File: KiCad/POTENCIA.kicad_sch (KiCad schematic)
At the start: 25 parts, among them J2 Screw_Terminal_01x02, J3 Screw_Terminal_01x02, J6 Screw_Terminal_01x02, SW7 SW_SPST, U2 LM2596S-5, U3 L298N, U7 LM1117DT-3.3

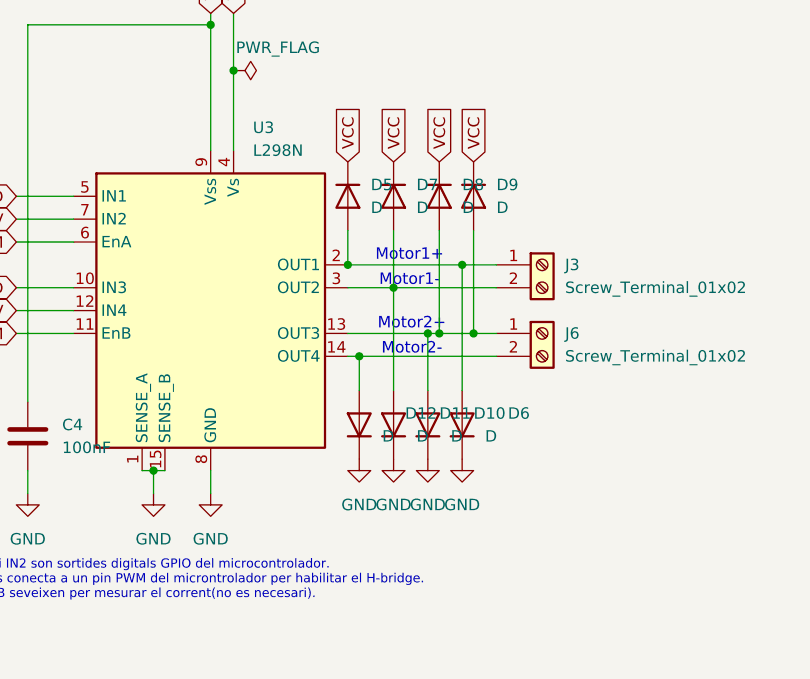
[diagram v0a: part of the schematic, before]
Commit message: a
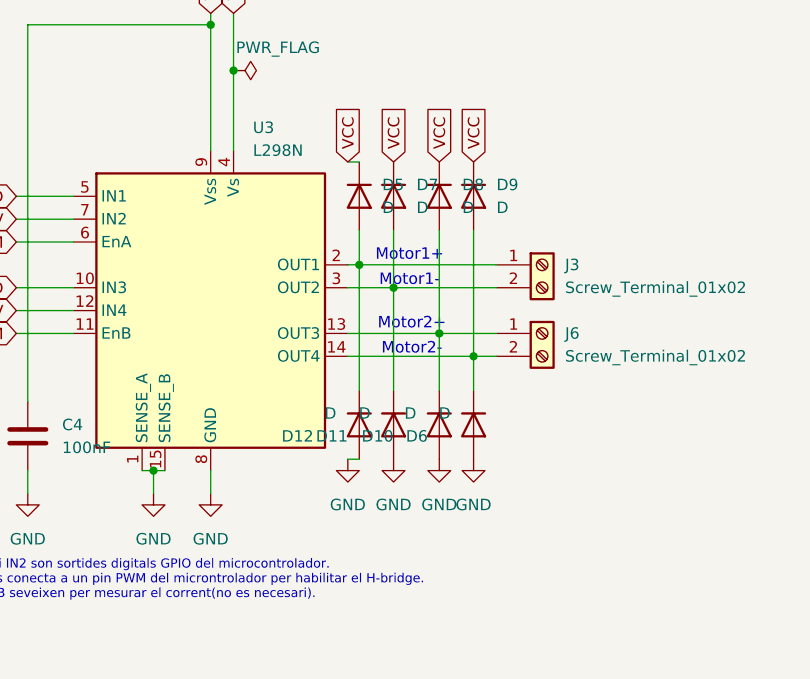
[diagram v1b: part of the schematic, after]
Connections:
- net GND: now also D10.2 (A), D11.2 (A), D12.2 (A), D6.2 (A); no longer D10.1 (K), D11.1 (K), D12.1 (K), D6.1 (K)
- net at D5.2 (A), J3.1 (Pin_1), U3.2 (OUT1): now also D12.1 (K); no longer D6.2 (A)
- net at D7.2 (A), J3.2 (Pin_2), U3.3 (OUT2): now also D11.1 (K); no longer D11.2 (A)
- net at J6.2 (Pin_2), U3.14 (OUT4): now also D6.1 (K), D9.2 (A); no longer D12.2 (A)
- net at D8.2 (A), J6.1 (Pin_1), U3.13 (OUT3): now also D10.1 (K); no longer D10.2 (A), D9.2 (A)
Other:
- moved on the sheet: D10, D11, D12, D5, D6
